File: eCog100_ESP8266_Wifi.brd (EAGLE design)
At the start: 48 x 28 mm, 11 parts

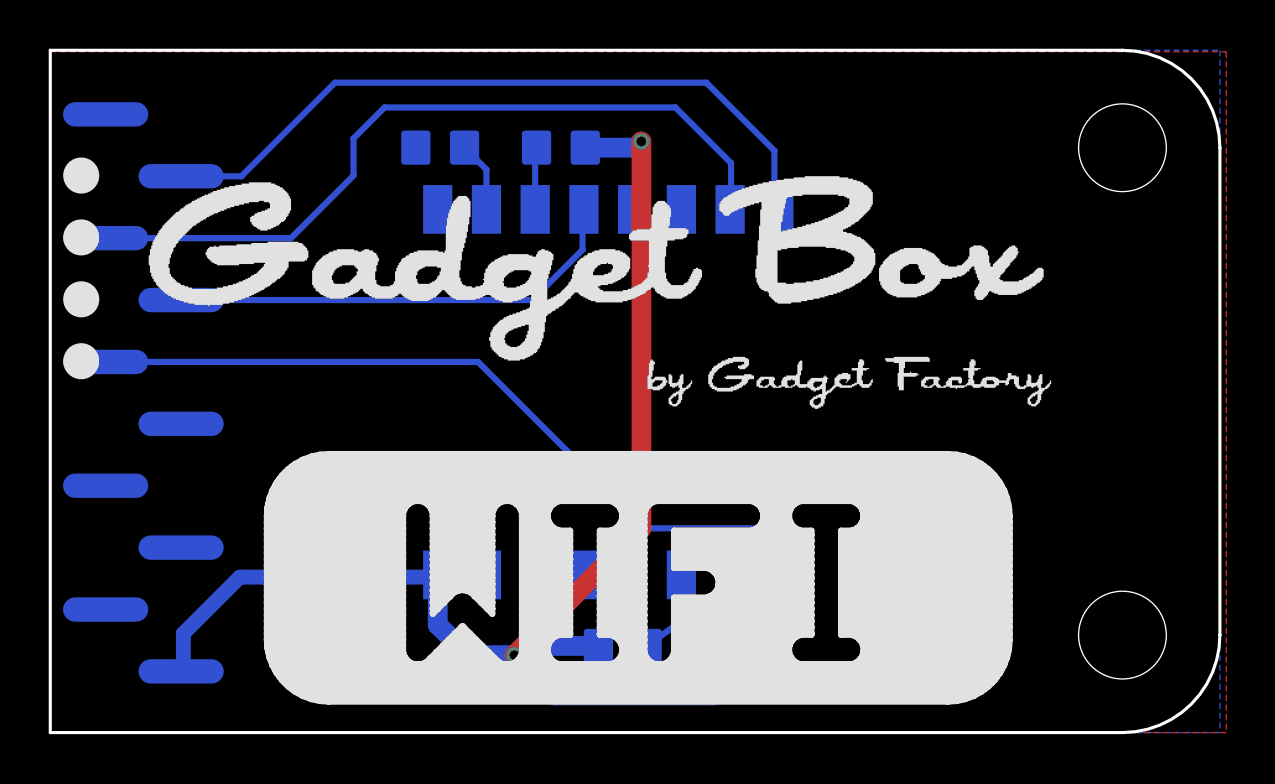
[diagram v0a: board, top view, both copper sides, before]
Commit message: Update all of the Fonts and graphics
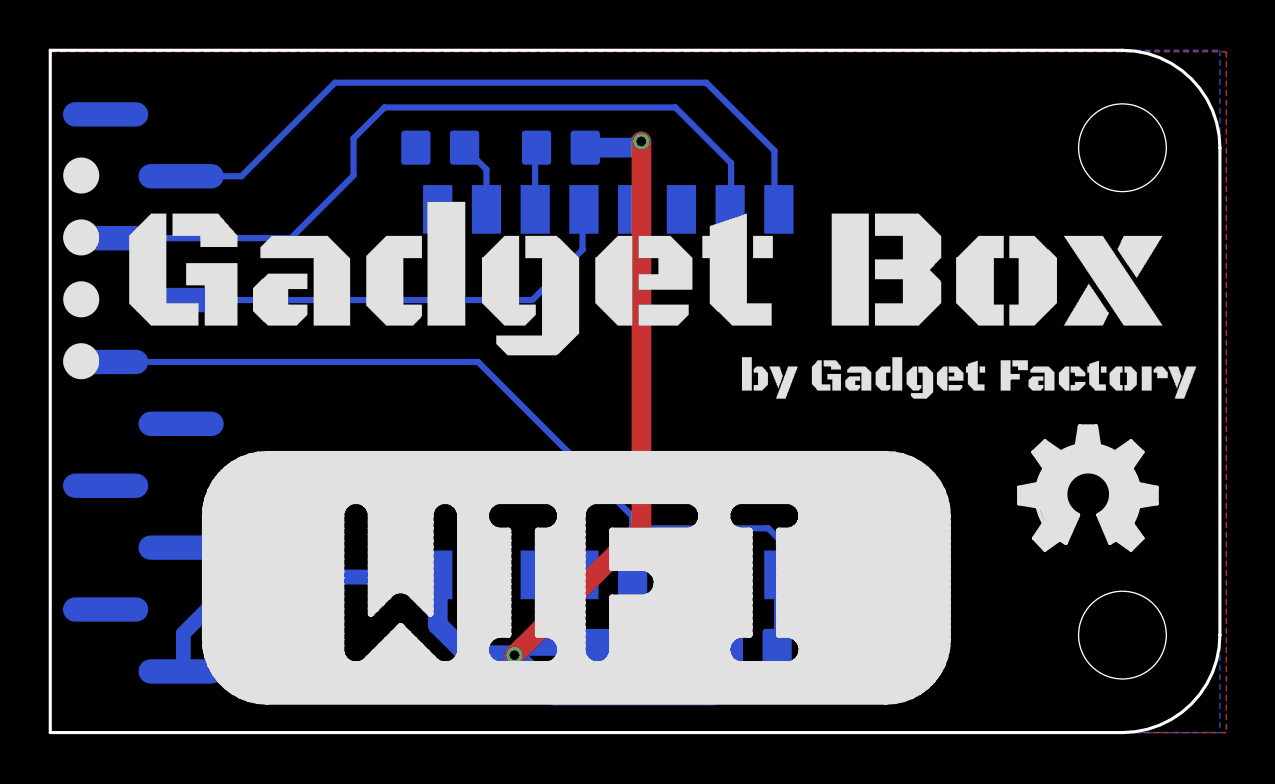
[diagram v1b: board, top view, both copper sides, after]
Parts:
- added U$6: (no value), ohw-logo:OSHW_FILLX200_NOTEXT
- moved U$1 1.77 mm to (24.5, 18.4)

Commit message: All the 2.0 updates
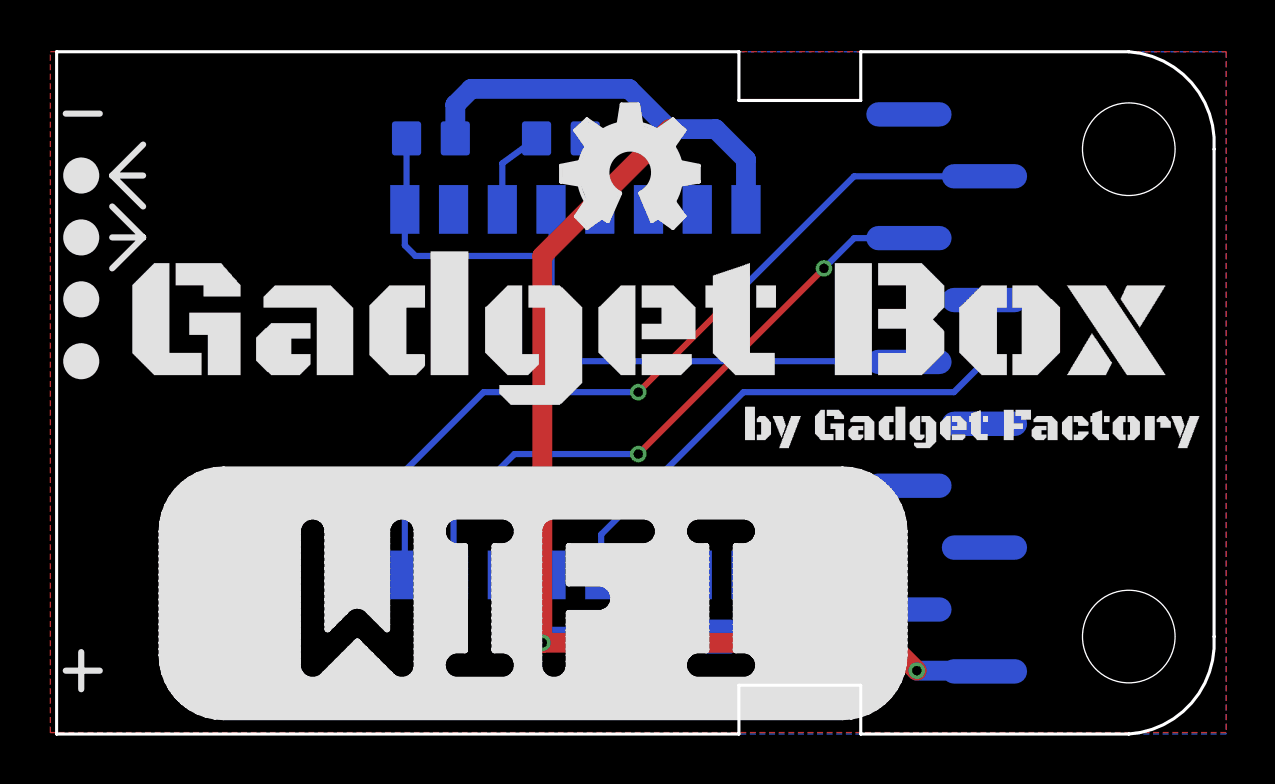
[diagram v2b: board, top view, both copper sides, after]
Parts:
- moved ECOG 55.8 mm to (48.3, 27.9), turned to 180 degrees
- moved R3 24.7 mm to (15.6, 24.4), turned to 180 degrees
- moved R2 23.6 mm to (28.4, 3.94), turned to 0 degrees
- moved U$6 23.0 mm to (21.0, 20.7)
- moved R4 21.0 mm to (21.0, 24.4), turned to 180 degrees
- moved R1 20.2 mm to (23.5, 3.94), turned to 0 degrees
- moved U$2 7.62 mm to (1.27, 15.2), turned to 180 degrees
- moved U$5 7.62 mm to (1.27, 22.9), turned to 180 degrees
- moved X1 6.35 mm to (19.1, 14.0), turned to 270 degrees
- moved U$3 2.54 mm to (1.27, 17.8), turned to 180 degrees
- moved U$4 2.54 mm to (1.27, 20.3), turned to 180 degrees
- moved U$1 2.04 mm to (24.6, 16.4)
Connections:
- net RX renamed RX/MOSI
- net TX renamed TX/MISO
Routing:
- net RESET: track 37.3 -> 30.9 mm
- net RX/MOSI: track 31.6 -> 25.9 mm, vias 0 -> 2
- net 3V3: track 59.1 -> 64.8 mm, vias 2 -> 3
- net GPIO0/BOOTLOAD: track 19.0 -> 22.9 mm
- net TX/MISO: track 29.6 -> 33.3 mm, vias 0 -> 2
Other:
- board size 48 x 28 mm -> 47.5 x 28 mm
- board text added: "0"
- board text added: "1"
- board text added: "2"
- board text added: "3"
- board text added: "RX/MOSI"
- board text added: "TX/MISO"
- board text added: "ecog100 v2.0"
- board text removed: "RX>"
- board text removed: "TX<"
- board text removed: "ecog100 v1.1"
